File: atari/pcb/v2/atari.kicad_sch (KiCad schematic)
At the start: 176 parts, among them J1 function_key_conn, J2 Conn_01x01_Pin, J3 function_key_conn, J4 Conn_01x01_Pin, J5 PowerLED, J6 Joysticks, SW1 RotaryEncoder_Switch, U1 Nice_Nano

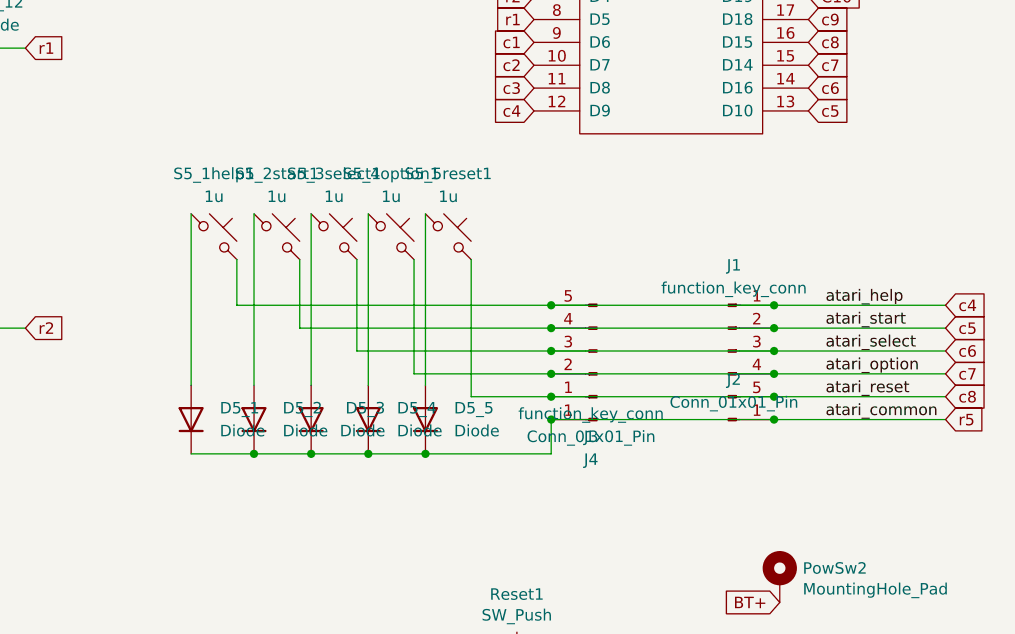
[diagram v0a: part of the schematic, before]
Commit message: fixed issues, added production file
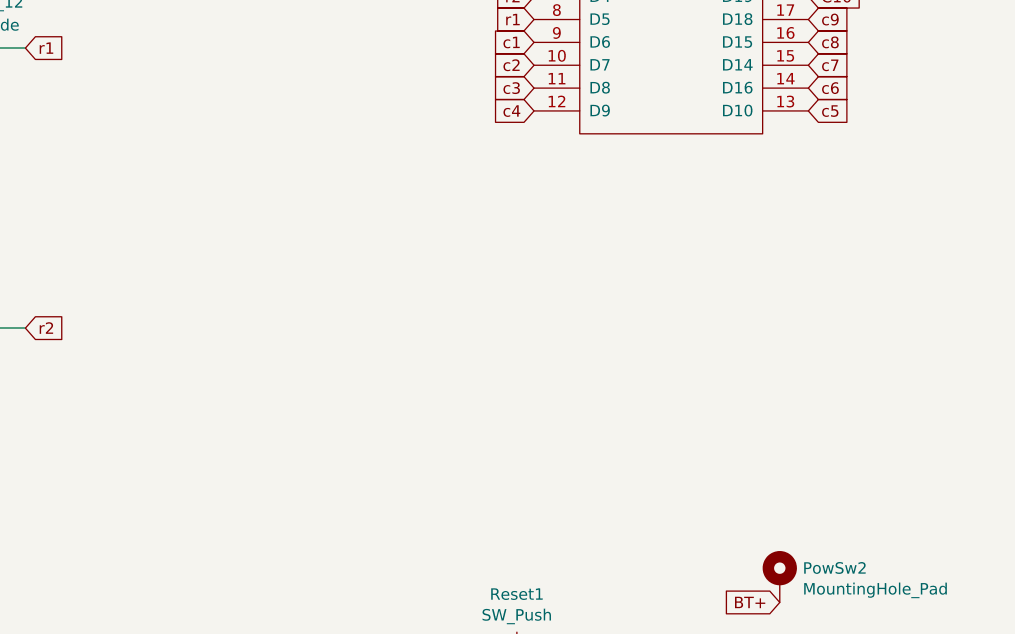
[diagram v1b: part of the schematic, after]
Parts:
- removed D5_1, D5_2, D5_3, D5_4, D5_5: Diode, ScottoKeebs_Components:Diode_DO-35, symbol ScottoKeebs:Placeholder_Diode
- removed J1, J3: function_key_conn, Connector_PinHeader_2.54mm:PinHeader_1x05_P2.54mm_Vertical, symbol Connector:Conn_01x05_Pin
- removed J2, J4: Conn_01x01_Pin, Connector_PinHeader_2.54mm:PinHeader_1x01_P2.54mm_Vertical, symbol Connector:Conn_01x01_Pin
- removed S5_1help1, S5_2start1, S5_3select1, S5_4option1, S5_5reset1: 1u, ScottoKeebs_MX:MX_PCB_1.00u, symbol ScottoKeebs:Placeholder_Keyswitch
